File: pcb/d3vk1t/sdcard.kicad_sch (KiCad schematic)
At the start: 9 parts, among them X2 Micro_SD_Card_Det

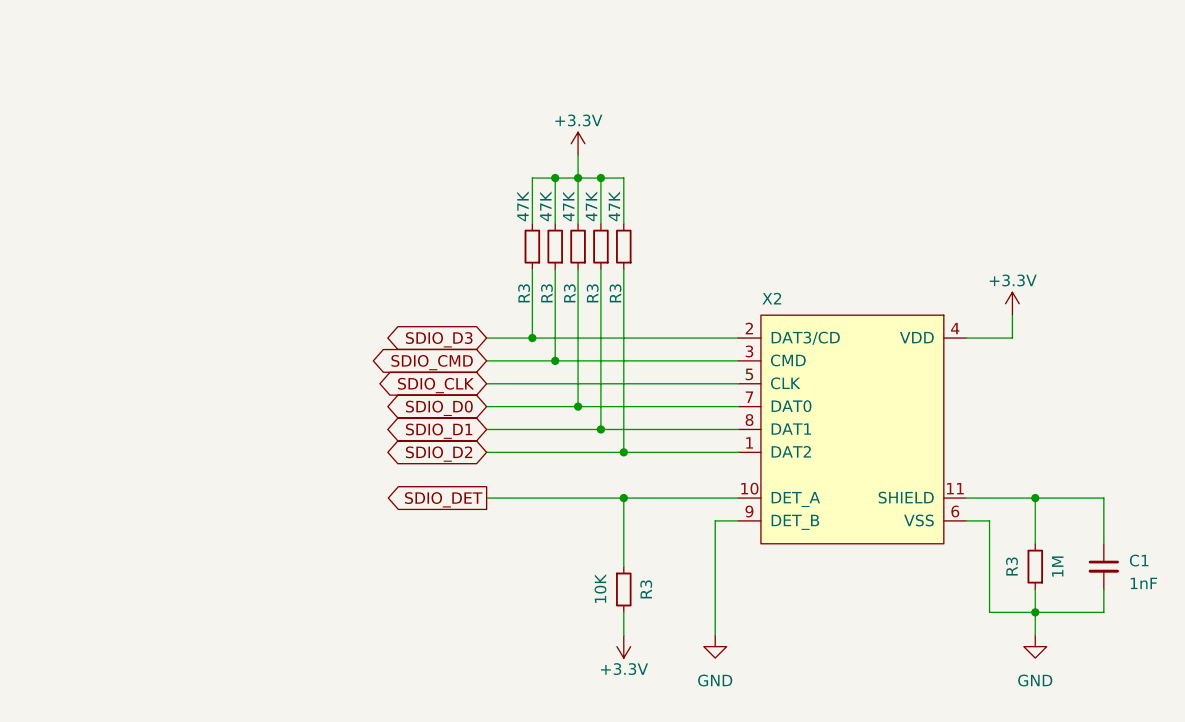
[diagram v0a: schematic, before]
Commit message: project update  - update pcb layout.  - update schmatics sheets.  - added manufacturing files.  - added documentation files.
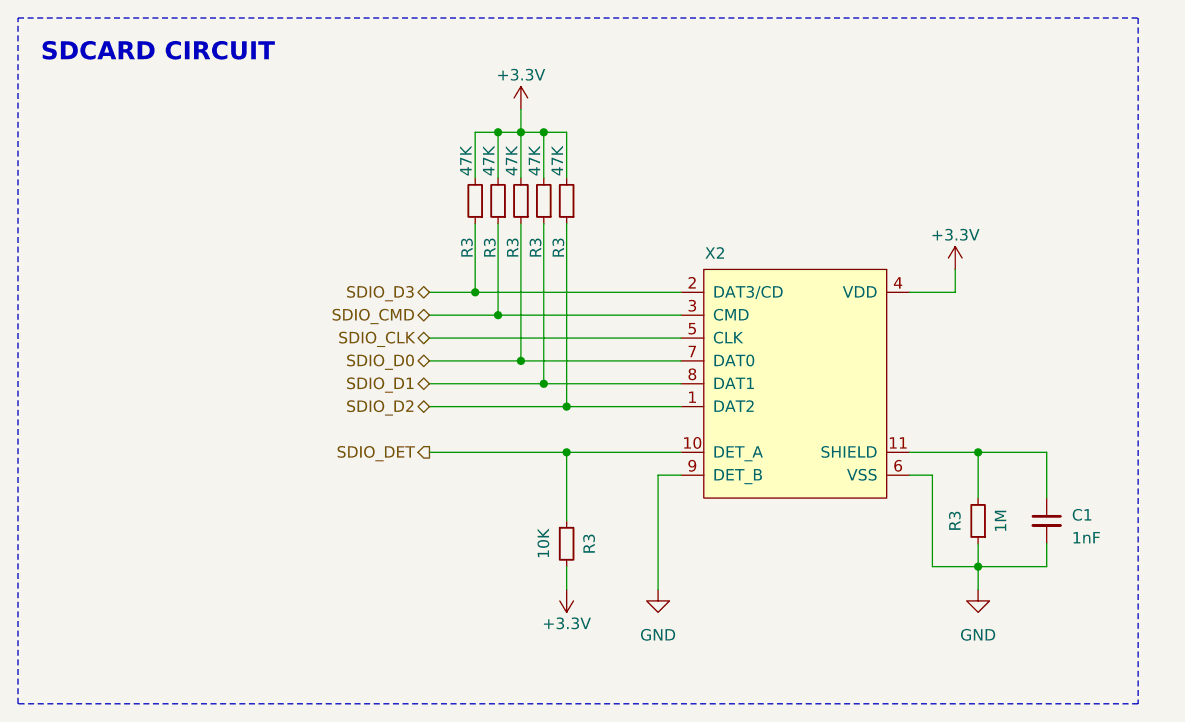
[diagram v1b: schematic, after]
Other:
- note added: "SDCARD CIRCUIT"
- title: (none) -> SDCard
- moved on the sheet: C1, R3, X2
